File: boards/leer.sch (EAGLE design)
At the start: 60 parts, among them IC1 XMEGA128A1, IC2 7805DT, Q1 BC846BSMD, Q2 BC846BSMD, Q3 BC846BSMD, Q4 BC846BSMD, Q5 BC846BSMD, Q6 BC846BSMD, Q7 BC846BSMD, Q8 BC846BSMD

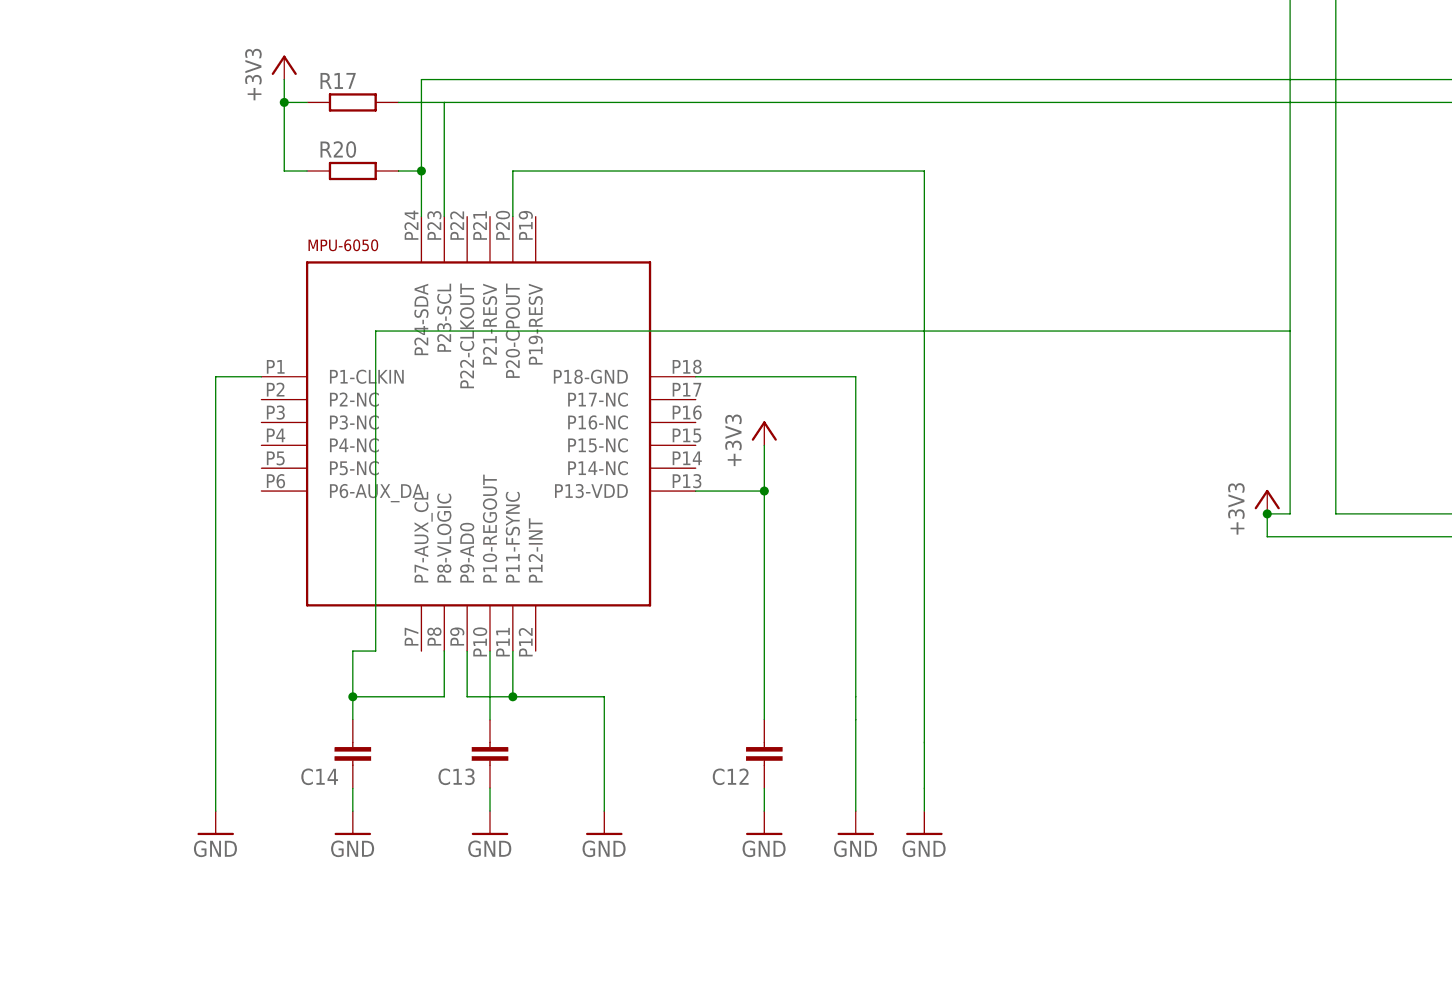
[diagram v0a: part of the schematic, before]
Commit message: Update layout
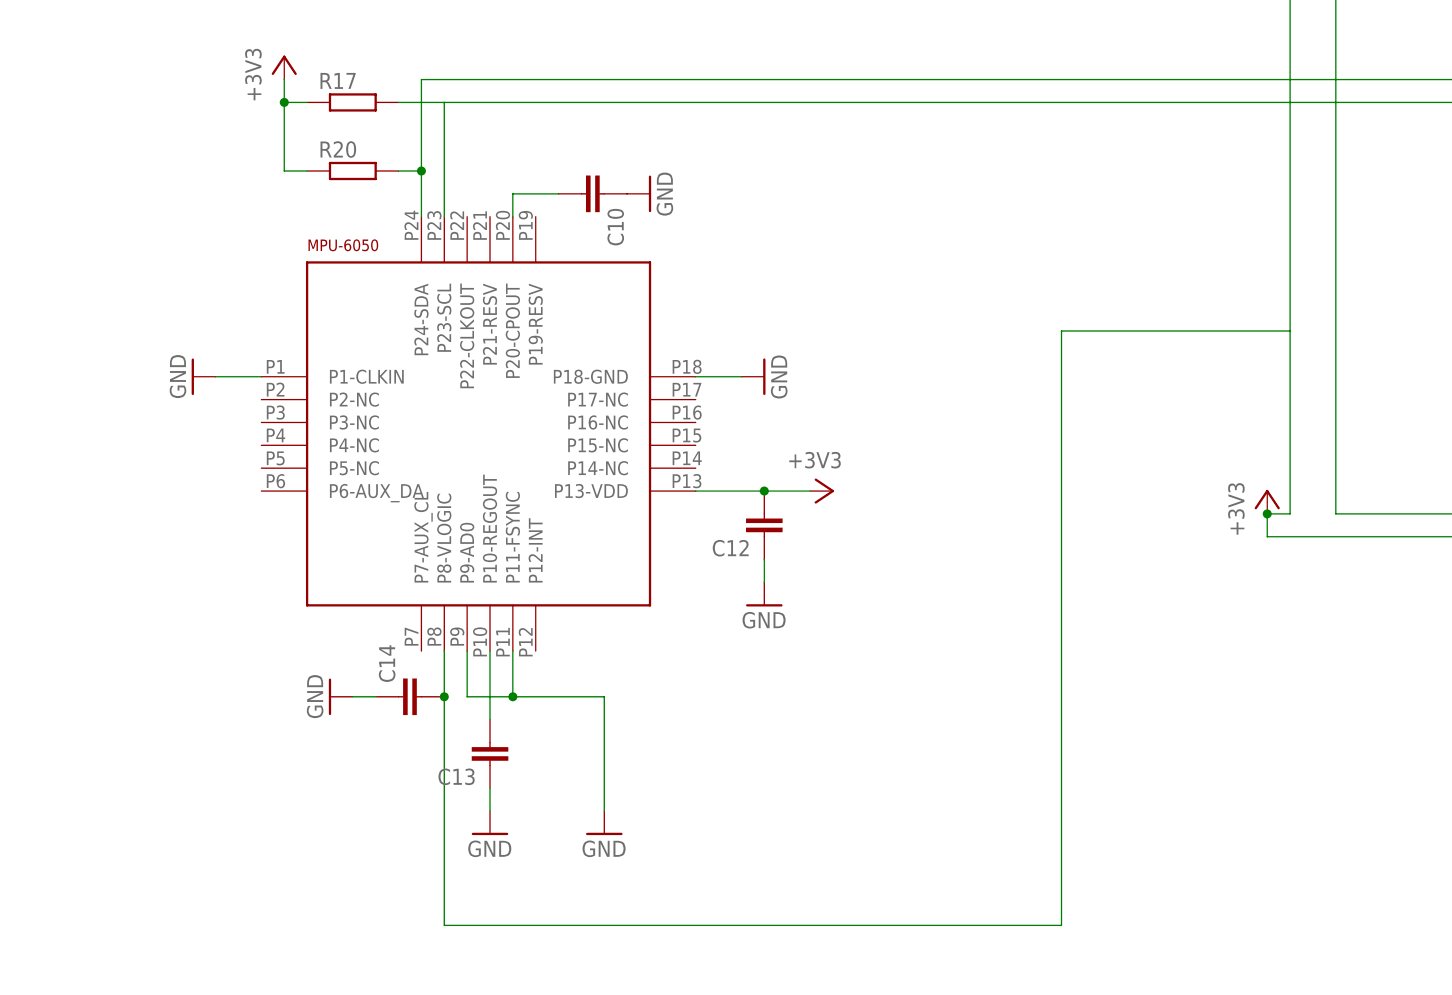
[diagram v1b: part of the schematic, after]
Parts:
- added C10: (no value), eagle-ltspice:CC0603
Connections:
- removed net N$38: U$3.P20-CPOUT
- new net N$35: C10.2, U$3.P20-CPOUT
- net GND: now also C10.1
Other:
- moved on the sheet: C12, C14
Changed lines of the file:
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@@
 <?xml version="1.0" encoding="utf-8"?>
 <!DOCTYPE eagle SYSTEM "eagle.dtd">
-<eagle version="6.5.0">
+<eagle version="6.4">
 <drawing>
 <settings>
@@
 <part name="R20" library="eagle-ltspice" deviceset="R" device="R0603"/>
 <part name="GND1" library="supply1" deviceset="GND" device=""/>
+<part name="C10" library="eagle-ltspice" deviceset="C" device="C0603"/>
 </parts>
 <sheets>
@@
 <instance part="U$3" gate="G$1" x="68.58" y="76.2"/>
 <instance part="+3V5" gate="G$1" x="45.72" y="119.38"/>
-<instance part="+3V6" gate="G$1" x="99.06" y="78.74"/>
-<instance part="GND12" gate="1" x="99.06" y="33.02"/>
-<instance part="GND13" gate="1" x="53.34" y="33.02"/>
+<instance part="+3V6" gate="G$1" x="106.68" y="71.12" rot="R270"/>
+<instance part="GND12" gate="1" x="99.06" y="58.42"/>
+<instance part="GND13" gate="1" x="50.8" y="48.26" rot="R270"/>
 <instance part="GND14" gate="1" x="68.58" y="33.02"/>
-<instance part="GND15" gate="1" x="116.84" y="33.02"/>
-<instance part="GND16" gate="1" x="38.1" y="33.02"/>
+<instance part="GND15" gate="1" x="86.36" y="104.14" rot="R90"/>
+<instance part="GND16" gate="1" x="35.56" y="83.82" rot="R270"/>
 <instance part="GND17" gate="1" x="81.28" y="33.02"/>
-<instance part="GND18" gate="1" x="109.22" y="33.02"/>
-<instance part="C12" gate="G$1" x="99.06" y="40.64" rot="R180"/>
+<instance part="GND18" gate="1" x="99.06" y="83.82" rot="R90"/>
+<instance part="C12" gate="G$1" x="99.06" y="66.04" rot="R180"/>
 <instance part="C13" gate="G$1" x="68.58" y="40.64" rot="R180"/>
-<instance part="C14" gate="G$1" x="53.34" y="40.64" rot="R180"/>
+<instance part="C14" gate="G$1" x="58.42" y="48.26" rot="R90"/>
 <instance part="+3V1" gate="G$1" x="154.94" y="71.12"/>
 <instance part="R17" gate="G$1" x="53.34" y="114.3"/>
 <instance part="R20" gate="G$1" x="53.34" y="106.68"/>
 <instance part="GND1" gate="1" x="289.56" y="66.04"/>
+<instance part="C10" gate="G$1" x="81.28" y="104.14" rot="R270"/>
 </instances>
 <busses>
@@
 <wire x1="91.44" y1="71.12" x2="99.06" y2="71.12" width="0.1524" layer="91"/>
 <pinref part="+3V6" gate="G$1" pin="+3V3"/>
-<wire x1="99.06" y1="71.12" x2="99.06" y2="76.2" width="0.1524" layer="91"/>
-<wire x1="99.06" y1="71.12" x2="99.06" y2="45.72" width="0.1524" layer="91"/>
+<wire x1="99.06" y1="71.12" x2="104.14" y2="71.12" width="0.1524" layer="91"/>
 <junction x="99.06" y="71.12"/>
 <pinref part="C12" gate="G$1" pin="2"/>
@@
 <pinref part="+3V1" gate="G$1" pin="+3V3"/>
 <junction x="154.94" y="68.58"/>
-<wire x1="53.34" y1="45.72" x2="53.34" y2="48.26" width="0.1524" layer="91"/>
-<wire x1="53.34" y1="48.26" x2="63.5" y2="48.26" width="0.1524" layer="91"/>
 <pinref part="U$3" gate="G$1" pin="P8-VLOGIC"/>
 <wire x1="63.5" y1="48.26" x2="63.5" y2="53.34" width="0.1524" layer="91"/>
-<wire x1="53.34" y1="48.26" x2="53.34" y2="53.34" width="0.1524" layer="91"/>
-<junction x="53.34" y="48.26"/>
+<wire x1="63.5" y1="48.26" x2="63.5" y2="22.86" width="0.1524" layer="91"/>
+<junction x="63.5" y="48.26"/>
 <pinref part="C14" gate="G$1" pin="2"/>
-<wire x1="53.34" y1="53.34" x2="55.88" y2="53.34" width="0.1524" layer="91"/>
-<wire x1="55.88" y1="53.34" x2="55.88" y2="88.9" width="0.1524" layer="91"/>
-<wire x1="55.88" y1="88.9" x2="157.48" y2="88.9" width="0.1524" layer="91"/>
+<wire x1="63.5" y1="22.86" x2="132.08" y2="22.86" width="0.1524" layer="91"/>
+<wire x1="132.08" y1="22.86" x2="132.08" y2="88.9" width="0.1524" layer="91"/>
+<wire x1="132.08" y1="88.9" x2="157.48" y2="88.9" width="0.1524" layer="91"/>
 </segment>
 </net>
 <net name="GND" class="0">
 <segment>
-<pinref part="GND15" gate="1" pin="GND"/>
-<wire x1="116.84" y1="38.1" x2="116.84" y2="35.56" width="0.1524" layer="91"/>
-</segment>
-<segment>
 <pinref part="GND12" gate="1" pin="GND"/>
-<wire x1="99.06" y1="38.1" x2="99.06" y2="35.56" width="0.1524" layer="91"/>
+<wire x1="99.06" y1="63.5" x2="99.06" y2="60.96" width="0.1524" layer="91"/>
 <pinref part="C12" gate="G$1" pin="1"/>
 </segment>
@@
 <segment>
 <pinref part="GND13" gate="1" pin="GND"/>
-<wire x1="53.34" y1="38.1" x2="53.34" y2="35.56" width="0.1524" layer="91"/>
+<wire x1="55.88" y1="48.26" x2="53.34" y2="48.26" width="0.1524" layer="91"/>
 <pinref part="C14" gate="G$1" pin="1"/>
 </segment>
@@
 <pinref part="U$3" gate="G$1" pin="P1-CLKIN"/>
 <wire x1="43.18" y1="83.82" x2="38.1" y2="83.82" width="0.1524" layer="91"/>
-<wire x1="38.1" y1="83.82" x2="38.1" y2="35.56" width="0.1524" layer="91"/>
 <pinref part="GND16" gate="1" pin="GND"/>
 </segment>
@@
 <pinref part="GND18" gate="1" pin="GND"/>
 <pinref part="U$3" gate="G$1" pin="P18-GND"/>
-<wire x1="91.44" y1="83.82" x2="109.22" y2="83.82" width="0.1524" layer="91"/>
-<wire x1="109.22" y1="83.82" x2="109.22" y2="48.26" width="0.1524" layer="91"/>
-<wire x1="109.22" y1="48.26" x2="109.22" y2="45.72" width="0.1524" layer="91"/>
-<wire x1="109.22" y1="45.72" x2="109.22" y2="35.56" width="0.1524" layer="91"/>
+<wire x1="91.44" y1="83.82" x2="96.52" y2="83.82" width="0.1524" layer="91"/>
 </segment>
 <segment>
@@
 <junction x="289.56" y="68.58"/>
 </segment>
+<segment>
+<pinref part="C10" gate="G$1" pin="1"/>
+<pinref part="GND15" gate="1" pin="GND"/>
+</segment>
 </net>
 <net name="N$37" class="0">
@@
 </segment>
 </net>
-<net name="N$38" class="0">
+<net name="N$35" class="0">
 <segment>
 <pinref part="U$3" gate="G$1" pin="P20-CPOUT"/>
-<wire x1="71.12" y1="101.6" x2="71.12" y2="106.68" width="0.1524" layer="91"/>
-<wire x1="71.12" y1="106.68" x2="116.84" y2="106.68" width="0.1524" layer="91"/>
-<wire x1="116.84" y1="106.68" x2="116.84" y2="43.18" width="0.1524" layer="91"/>
-<wire x1="116.84" y1="43.18" x2="116.84" y2="38.1" width="0.1524" layer="91"/>
-</segment>
-</net>
+<pinref part="C10" gate="G$1" pin="2"/>
+<wire x1="71.12" y1="101.6" x2="71.12" y2="104.14" width="0.1524" layer="91"/>
+<wire x1="71.12" y1="104.14" x2="76.2" y2="104.14" width="0.1524" layer="91"/>
+</segment>
+</net>
